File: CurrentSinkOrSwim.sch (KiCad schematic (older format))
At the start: 4 parts, among them P101 ext pwr, P102 pwr sel, P103 Input, P4 Gnd

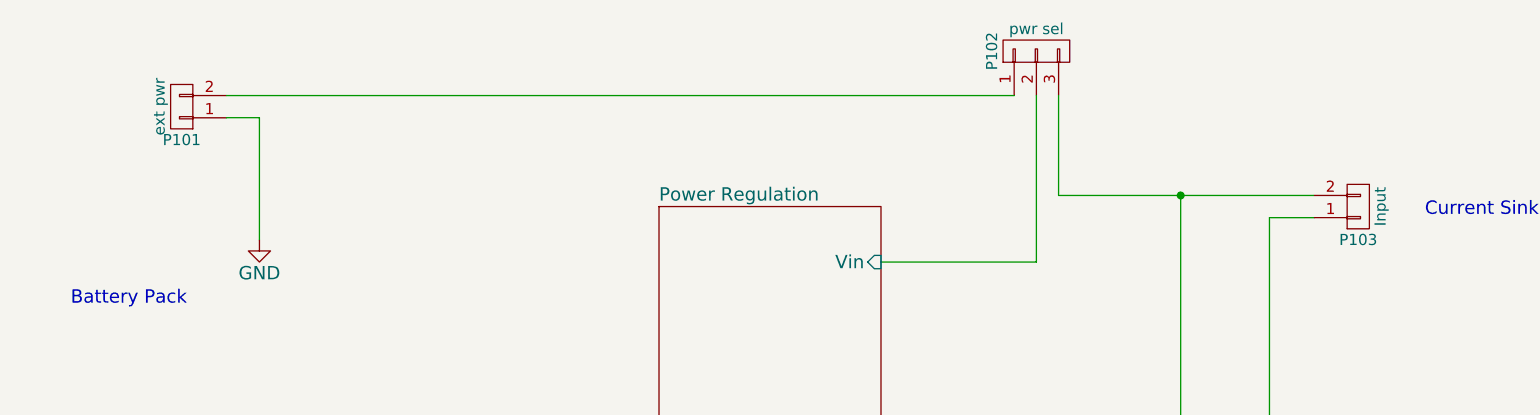
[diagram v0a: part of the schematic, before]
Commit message: test netlist
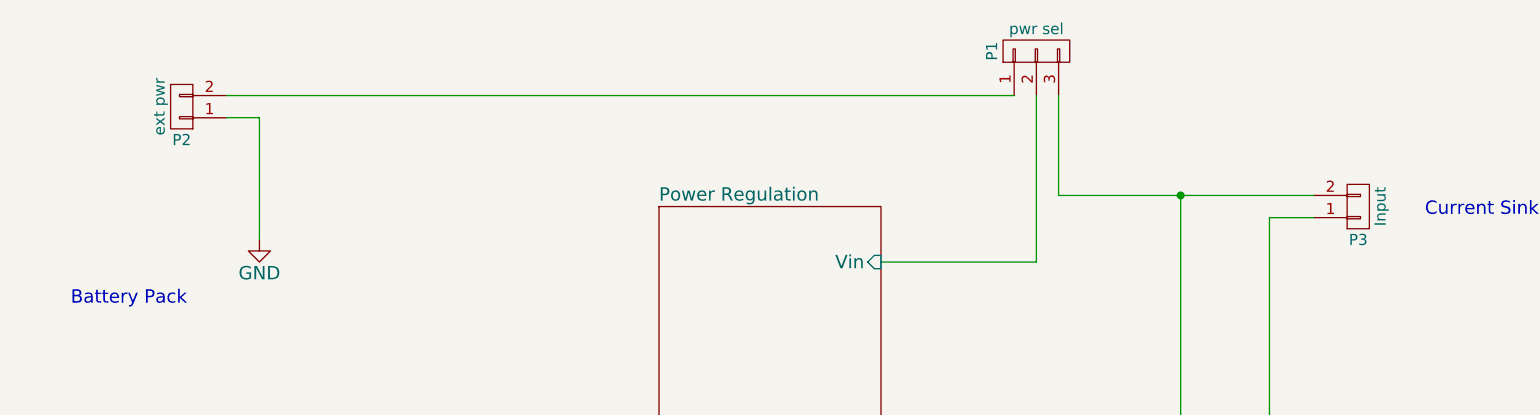
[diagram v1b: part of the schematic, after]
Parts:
- renumbered P102 to P1, P101 to P2, P103 to P3
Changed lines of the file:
@@
 $EndDescr
 $Comp
-L CONN_01X02 P103
+L CONN_01X02 P3
 U 1 1 54CEA02B
 P 8300 1300
-F 0 "P103" H 8300 1450 50  0000 C CNN
+F 0 "P3" H 8300 1450 50  0000 C CNN
 F 1 "Input" V 8400 1300 50  0000 C CNN
 F 2 "Current:TB-01x02" H 8300 1300 60  0001 C CNN
@@
 $EndComp
 $Comp
-L CONN_01X03 P102
+L CONN_01X03 P1
 U 1 1 54D855F7
 P 6850 600
-F 0 "P102" H 6850 800 50  0000 C CNN
+F 0 "P1" H 6850 800 50  0000 C CNN
 F 1 "pwr sel" V 6950 600 50  0000 C CNN
 F 2 "Pin_Headers:Pin_Header_Straight_1x03" H 6850 600 60  0001 C CNN
@@
 $EndComp
 $Comp
-L CONN_01X02 P101
+L CONN_01X02 P2
 U 1 1 54D858EB
 P 3000 850
-F 0 "P101" H 3000 1000 50  0000 C CNN
+F 0 "P2" H 3000 1000 50  0000 C CNN
 F 1 "ext pwr" V 3100 850 50  0000 C CNN
 F 2 "Current:Pads-01x02" H 3000 850 60  0001 C CNN
@@
 $EndComp
 $Comp
-L GND #PWR01
+L GND #PWR1
 U 1 1 54D85A15
 P 3350 1450
-F 0 "#PWR01" H 3350 1200 60  0001 C CNN
+F 0 "#PWR1" H 3350 1200 60  0001 C CNN
 F 1 "GND" H 3350 1300 60  0000 C CNN
 F 2 "" H 3350 1450 60  0000 C CNN
@@
 	4550 4400 4800 4400
 $Comp
-L GND #PWR02
+L GND #PWR3
 U 1 1 54DB4AD2
 P 7900 6250
-F 0 "#PWR02" H 7900 6000 60  0001 C CNN
+F 0 "#PWR3" H 7900 6000 60  0001 C CNN
 F 1 "GND" H 7900 6100 60  0000 C CNN
 F 2 "" H 7900 6250 60  0000 C CNN
@@
 $EndComp
 $Comp
-L GND #PWR03
+L GND #PWR2
 U 1 1 54F1F7D2
 P 2200 4350
-F 0 "#PWR03" H 2200 4100 60  0001 C CNN
+F 0 "#PWR2" H 2200 4100 60  0001 C CNN
 F 1 "GND" H 2200 4200 60  0000 C CNN
 F 2 "" H 2200 4350 60  0000 C CNN

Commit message: Routing done - Final
Just add artwork
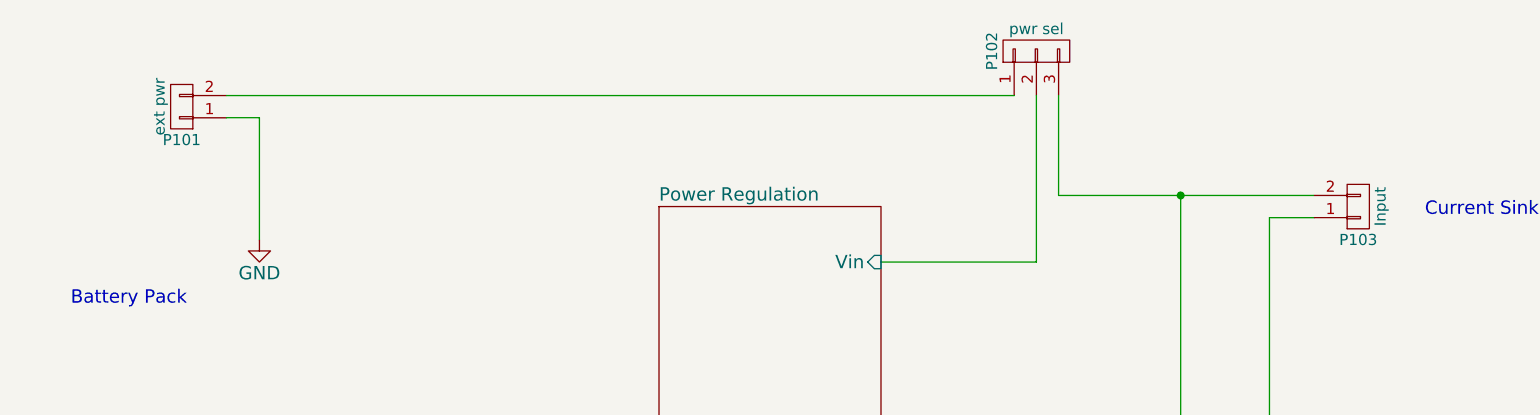
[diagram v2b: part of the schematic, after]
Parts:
- renumbered P2 to P101, P1 to P102, P3 to P103
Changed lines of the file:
@@
 $EndDescr
 $Comp
-L CONN_01X02 P3
+L CONN_01X02 P103
 U 1 1 54CEA02B
 P 8300 1300
-F 0 "P3" H 8300 1450 50  0000 C CNN
+F 0 "P103" H 8300 1450 50  0000 C CNN
 F 1 "Input" V 8400 1300 50  0000 C CNN
 F 2 "Current:TB-01x02" H 8300 1300 60  0001 C CNN
@@
 $EndComp
 $Comp
-L CONN_01X03 P1
+L CONN_01X03 P102
 U 1 1 54D855F7
 P 6850 600
-F 0 "P1" H 6850 800 50  0000 C CNN
+F 0 "P102" H 6850 800 50  0000 C CNN
 F 1 "pwr sel" V 6950 600 50  0000 C CNN
 F 2 "Pin_Headers:Pin_Header_Straight_1x03" H 6850 600 60  0001 C CNN
@@
 $EndComp
 $Comp
-L CONN_01X02 P2
+L CONN_01X02 P101
 U 1 1 54D858EB
 P 3000 850
-F 0 "P2" H 3000 1000 50  0000 C CNN
+F 0 "P101" H 3000 1000 50  0000 C CNN
 F 1 "ext pwr" V 3100 850 50  0000 C CNN
 F 2 "Current:Pads-01x02" H 3000 850 60  0001 C CNN
@@
 $EndComp
 $Comp
-L GND #PWR1
+L GND #PWR01
 U 1 1 54D85A15
 P 3350 1450
-F 0 "#PWR1" H 3350 1200 60  0001 C CNN
+F 0 "#PWR01" H 3350 1200 60  0001 C CNN
 F 1 "GND" H 3350 1300 60  0000 C CNN
 F 2 "" H 3350 1450 60  0000 C CNN
@@
 	4550 4400 4800 4400
 $Comp
-L GND #PWR3
+L GND #PWR02
 U 1 1 54DB4AD2
 P 7900 6250
-F 0 "#PWR3" H 7900 6000 60  0001 C CNN
+F 0 "#PWR02" H 7900 6000 60  0001 C CNN
 F 1 "GND" H 7900 6100 60  0000 C CNN
 F 2 "" H 7900 6250 60  0000 C CNN
@@
 $EndComp
 $Comp
-L GND #PWR2
+L GND #PWR03
 U 1 1 54F1F7D2
 P 2200 4350
-F 0 "#PWR2" H 2200 4100 60  0001 C CNN
+F 0 "#PWR03" H 2200 4100 60  0001 C CNN
 F 1 "GND" H 2200 4200 60  0000 C CNN
 F 2 "" H 2200 4350 60  0000 C CNN
